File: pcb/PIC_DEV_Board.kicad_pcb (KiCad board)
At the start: 2 copper layers, 25.5 x 47.5 mm, 8 parts, among them J1 Conn_01x08_Pin, J3 Conn_01x15_Pin, J4 Conn_01x02_Pin

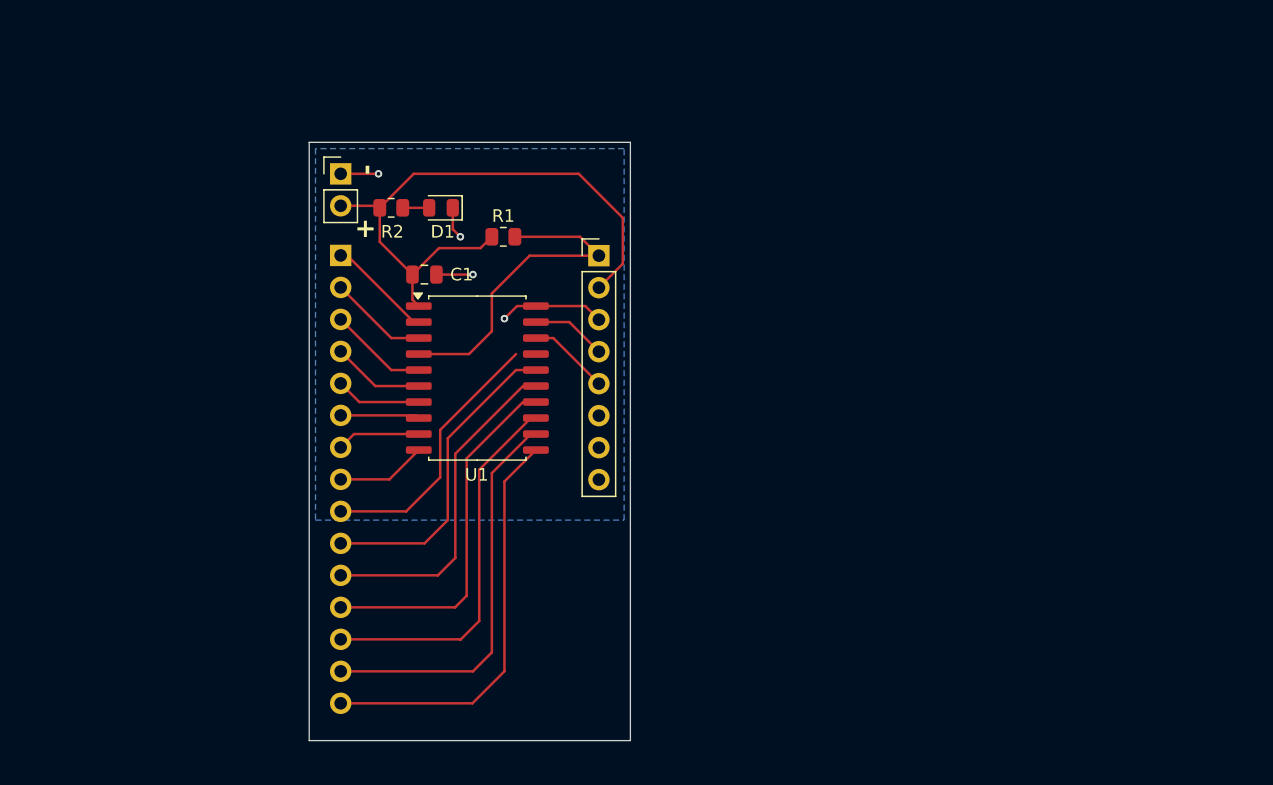
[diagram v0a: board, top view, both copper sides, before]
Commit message: higher functionality board
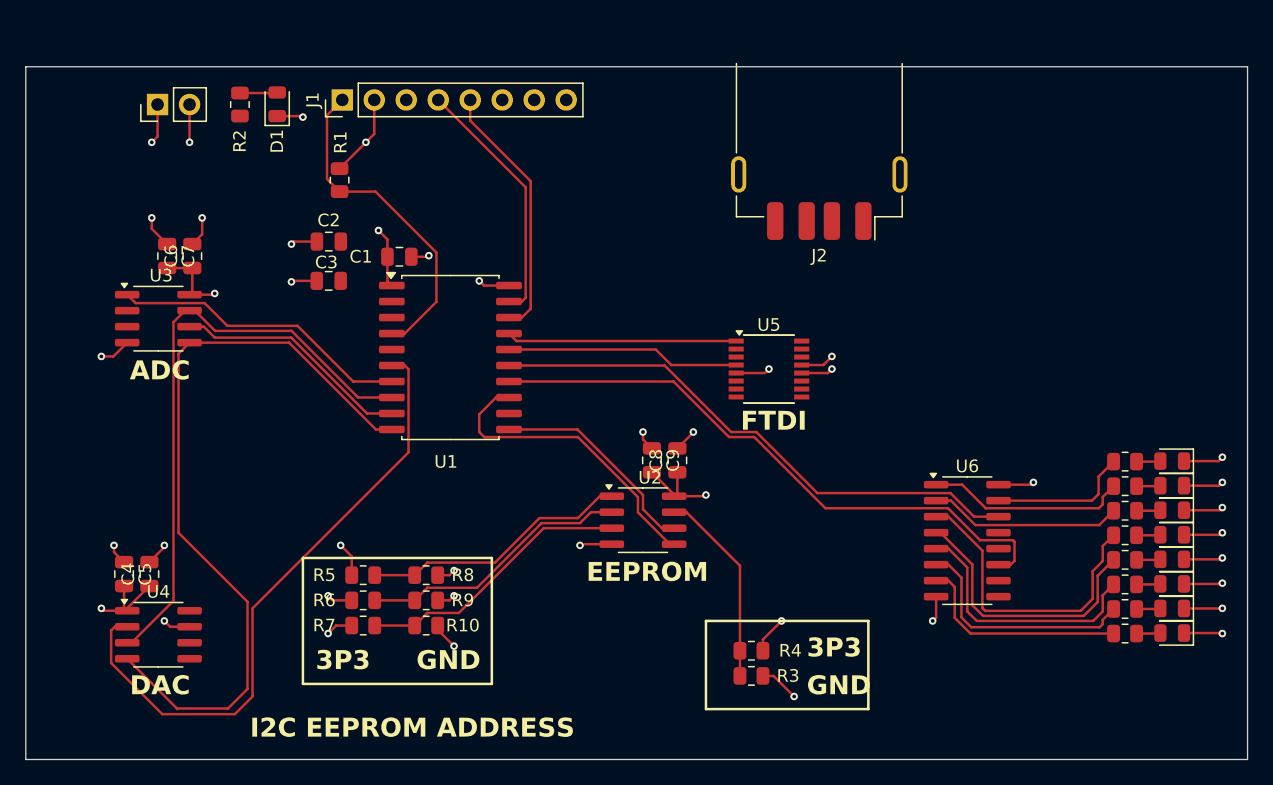
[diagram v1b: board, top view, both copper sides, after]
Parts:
- removed J3: Conn_01x15_Pin, Connector_PinHeader_2.54mm:PinHeader_1x15_P2.54mm_Vertical
- added C2: 30pF, Capacitor_SMD:C_0805_2012Metric, F.Cu at (136.1, 91.9)
- added C3: 30pF, Capacitor_SMD:C_0805_2012Metric, F.Cu at (136.1, 95.0)
- added C4: 0.1uF, Capacitor_SMD:C_0805_2012Metric, F.Cu at (121.8, 118.3)
- added C5: 10uF, Capacitor_SMD:C_0805_2012Metric, F.Cu at (119.8, 118.3)
- added C6: 0.1uF, Capacitor_SMD:C_0805_2012Metric, F.Cu at (125.2, 93.0)
- added C7: 10uF, Capacitor_SMD:C_0805_2012Metric, F.Cu at (123.2, 93.0)
- added C8: 0.1uF, Capacitor_SMD:C_0805_2012Metric, F.Cu at (163.7, 109.2)
- added C9: 10uF, Capacitor_SMD:C_0805_2012Metric, F.Cu at (161.7, 109.2)
- added D2: LED, LED_SMD:LED_0805_2012Metric, F.Cu at (203.0, 109.3)
- added D3: LED, LED_SMD:LED_0805_2012Metric, F.Cu at (203.0, 111.3)
- added D4: LED, LED_SMD:LED_0805_2012Metric, F.Cu at (203.0, 113.2)
- added D5: LED, LED_SMD:LED_0805_2012Metric, F.Cu at (203.0, 115.2)
- added D6: LED, LED_SMD:LED_0805_2012Metric, F.Cu at (203.0, 117.1)
- added D7: LED, LED_SMD:LED_0805_2012Metric, F.Cu at (203.0, 119.1)
- added D8: LED, LED_SMD:LED_0805_2012Metric, F.Cu at (203.0, 121.0)
- added D9: LED, LED_SMD:LED_0805_2012Metric, F.Cu at (203.0, 123.0)
- added J2: USB_A, Connector_USB:USB_A_Receptacle_GCT_USB1046, F.Cu at (175.0, 83.0)
- added R10: 10K, Resistor_SMD:R_0805_2012Metric, F.Cu at (143.8, 122.4)
- added R11: 560, Resistor_SMD:R_0805_2012Metric, F.Cu at (199.3, 109.3)
- added R12: 560, Resistor_SMD:R_0805_2012Metric, F.Cu at (199.3, 111.3)
- added R13: 560, Resistor_SMD:R_0805_2012Metric, F.Cu at (199.3, 113.2)
- added R14: 560, Resistor_SMD:R_0805_2012Metric, F.Cu at (199.3, 115.2)
- added R15: 560, Resistor_SMD:R_0805_2012Metric, F.Cu at (199.3, 117.2)
- added R16: 560, Resistor_SMD:R_0805_2012Metric, F.Cu at (199.3, 119.1)
- added R17: 560, Resistor_SMD:R_0805_2012Metric, F.Cu at (199.3, 121.0)
- added R18: 560, Resistor_SMD:R_0805_2012Metric, F.Cu at (199.3, 123.0)
- added R3: 0, Resistor_SMD:R_0805_2012Metric, F.Cu at (169.6, 126.4)
- added R4: 10K, Resistor_SMD:R_0805_2012Metric, F.Cu at (169.6, 124.4)
- added R5: 10K, Resistor_SMD:R_0805_2012Metric, F.Cu at (138.8, 118.4)
- added R6: 10K, Resistor_SMD:R_0805_2012Metric, F.Cu at (138.8, 120.4)
- added R7: 10K, Resistor_SMD:R_0805_2012Metric, F.Cu at (138.8, 122.4)
- added R8: 10K, Resistor_SMD:R_0805_2012Metric, F.Cu at (143.8, 118.4)
- added R9: 10K, Resistor_SMD:R_0805_2012Metric, F.Cu at (143.8, 120.4)
- added U2: ~, Package_SO:SOIC-8_3.9x4.9mm_P1.27mm, F.Cu at (161.0, 114.0)
- added U3: MCP3002, Package_SO:SOIC-8_3.9x4.9mm_P1.27mm, F.Cu at (122.5, 98.0)
- added U4: MCP4801, Package_SO:SOIC-8_3.9x4.9mm_P1.27mm, F.Cu at (122.5, 123.1)
- added U5: FT230XS, Package_SO:SSOP-16_3.9x4.9mm_P0.635mm, F.Cu at (171.0, 102.0)
- added U6: 74HC595, Package_SO:SOIC-16_3.9x9.9mm_P1.27mm, F.Cu at (186.8, 115.6)
- moved J1 23.8 mm to (137.1, 80.6), turned to 90 degrees
- moved J4 15.5 mm to (122.5, 81.0), turned to 90 degrees
- moved D1 15.4 mm to (132.0, 81.0), turned to 90 degrees
- moved R2 14.5 mm to (129.0, 81.0), turned to 90 degrees
- moved R1 13.8 mm to (136.9, 87.0), turned to -90 degrees
- moved U1 2.69 mm to (145.7, 101.1)
- moved C1 2.44 mm to (141.7, 93.1)
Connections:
- net Net-(J1-Pin_1) renamed /Vpp/RA3/MCLR
- net Net-(J1-Pin_2) renamed +3V3
- U1 pad 10: Net-(J3-Pin_8) -> /SDI
- U1 pad 12: Net-(J3-Pin_14) -> unconnected-(U1-RB5-Pad12)
- U1 pad 5: Net-(J3-Pin_3) -> unconnected-(U1-RC5-Pad5)
- U1 pad 6: Net-(J3-Pin_4) -> /~{DAC_CS}
- U1 pad 7: Net-(J3-Pin_5) -> /~{ADC_CS}
- U1 pad 8: Net-(J3-Pin_6) -> /SCK
- U1 pad 9: Net-(J3-Pin_7) -> /SDO
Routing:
- net /SDI: track 0.00 -> 60.9 mm
- net Earth: track 16.8 -> 73.0 mm, vias 4 -> 30
- net /~{DAC_CS}: track 0.00 -> 50.0 mm
- net /SCK: track 0.00 -> 47.7 mm
- net Net-(J3-Pin_14): track 31.6 -> 0.00 mm
- net Net-(U6-QD): track 0.00 -> 24.3 mm
- net /~{ADC_CS}: track 0.00 -> 23.9 mm
- net Net-(U2-A2): track 0.00 -> 22.0 mm
- net Net-(U6-QE): track 0.00 -> 21.8 mm
- net Net-(U2-A1): track 0.00 -> 21.7 mm
- net Net-(U2-A0): track 0.00 -> 21.4 mm
- net Net-(U6-QF): track 0.00 -> 20.5 mm
- net Net-(U1-RC2): track 28.6 -> 48.3 mm
- net /SDO: track 0.00 -> 18.9 mm
- net Net-(U6-QG): track 0.00 -> 18.8 mm
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- added copper zone on In2.Cu, net +3V3
- added copper zone on In1.Cu, net Earth
- removed copper zone on B.Cu, net Earth
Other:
- board size 25.5 x 47.5 mm -> 97 x 55 mm
- copper layers 2 -> 4
- board text added: "3P3"
- board text added: "ADC"
- board text added: "DAC"
- board text added: "EEPROM"
- board text added: "FTDI"
- board text added: "GND"
- board text added: "I2C EEPROM ADDRESS"
- board text removed: "+"
- board text removed: "-"

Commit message: size reduction
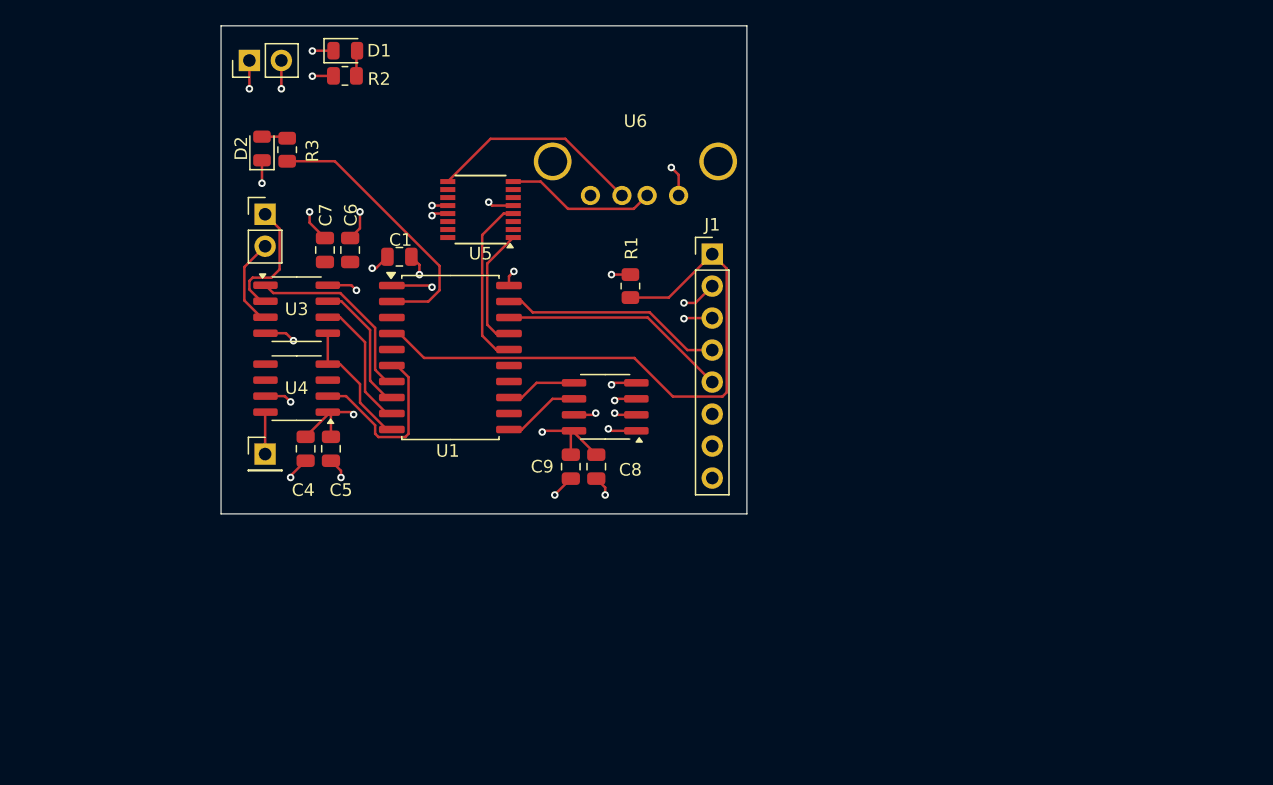
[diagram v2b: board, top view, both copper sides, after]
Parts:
- removed C2, C3: 30pF, Capacitor_SMD:C_0805_2012Metric
- removed D3, D4, D5, D6, D7, D8, D9: LED, LED_SMD:LED_0805_2012Metric
- removed J2: USB_A, Connector_USB:USB_A_Receptacle_GCT_USB1046
- removed R10, R4, R5, R6, R7, R8, R9: 10K, Resistor_SMD:R_0805_2012Metric
- removed R11, R12, R13, R14, R15, R16, R17, R18: 560, Resistor_SMD:R_0805_2012Metric
- added J3: Conn_01x02_Pin, Connector_PinHeader_2.54mm:PinHeader_1x02_P2.54mm_Vertical, F.Cu at (131.0, 89.7)
- added J5: Conn_01x01_Pin, Connector_PinHeader_2.54mm:PinHeader_1x01_P2.54mm_Vertical, F.Cu at (131.0, 108.8)
- R3: value 0 -> 1K
- U6: value 74HC595 -> ~; footprint Package_SO:SOIC-16_3.9x9.9mm_P1.27mm -> myCustomFootprints:USB-A1HSB6
- moved D2 76.4 mm to (130.8, 84.5), turned to 90 degrees
- moved R3 55.7 mm to (132.8, 84.6), turned to 90 degrees
- moved U6 38.1 mm to (160.3, 88.2), turned to 180 degrees
- moved J1 31.8 mm to (166.5, 92.9), turned to 0 degrees
- moved U5 26.2 mm to (148.1, 89.3), turned to 180 degrees
- moved R1 24.6 mm to (160.0, 95.4)
- moved U4 22.4 mm to (133.5, 103.5), turned to 180 degrees
- moved C5 19.2 mm to (136.2, 108.3), turned to 90 degrees
- moved C4 15.9 mm to (134.2, 108.3), turned to -90 degrees
- moved C6 12.5 mm to (137.8, 92.5)
- moved C7 12.5 mm to (135.8, 92.5)
- moved U3 11.0 mm to (133.5, 97.2)
- moved U2 9.49 mm to (158.0, 105.0), turned to 180 degrees
- moved R2 8.64 mm to (137.3, 78.7), turned to 0 degrees
- moved C8 8.47 mm to (155.3, 109.8), turned to -90 degrees
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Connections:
- R3 pad 1: Earth -> Net-(U1-RA5)
- R3 pad 2: Net-(U2-WP) -> Net-(D2-A)
- U1 pad 14: Net-(U1-RC2) -> unconnected-(U1-RC2-Pad14)
- U1 pad 15: Net-(U1-RC1) -> unconnected-(U1-RC1-Pad15)
- U1 pad 3: Net-(U1-RA4) -> unconnected-(U1-RA4-Pad3)
- U2 pad 1: Net-(U2-A0) -> Earth
- U2 pad 2: Net-(U2-A1) -> Earth
- U2 pad 3: Net-(U2-A2) -> Earth
- U2 pad 7: Net-(U2-WP) -> Earth
- U3 pad 2: unconnected-(U3-CH0-Pad2) -> Net-(J3-Pin_1)
- U3 pad 3: unconnected-(U3-CH1-Pad3) -> Net-(J3-Pin_2)
- U4 pad 8: unconnected-(U4-Vout-Pad8) -> Net-(J5-Pin_1)
- U5 pad 8: Net-(J2-D+) -> Net-(U5-USBDP)
- U5 pad 9: Net-(J2-D-) -> Net-(U5-USBDM)
- U6 pad 1: Net-(U6-QB) -> unconnected-(U6-VCC-Pad1)
- U6 pad 2: Net-(U6-QC) -> Net-(U5-USBDM)
- U6 pad 3: Net-(U6-QD) -> Net-(U5-USBDP)
- U6 pad 4: Net-(U6-QE) -> Earth
- U6 pad 5: Net-(U6-QF) -> (no net)
- U6 pad 6: Net-(U6-QG) -> (no net)
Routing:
- net /SDI: track 60.9 -> 10.6 mm
- net Net-(U1-RC2): track 48.3 -> 0.00 mm
- net Net-(U1-RC1): track 43.8 -> 0.00 mm
- net /SCK: track 47.7 -> 10.6 mm
- net /~{DAC_CS}: track 50.0 -> 14.5 mm
- net Earth: track 73.0 -> 43.1 mm, vias 30 -> 22
- net Net-(U6-QD): track 24.3 -> 0.00 mm
- net Net-(U2-A2): track 22.0 -> 0.00 mm
- net /Vpp/RA3/MCLR: track 26.4 -> 48.2 mm
- net Net-(U6-QE): track 21.8 -> 0.00 mm
- net Net-(U2-A1): track 21.7 -> 0.00 mm
- net Net-(U1-RA5): track 0.00 -> 21.6 mm
- net Net-(U2-A0): track 21.4 -> 0.00 mm
- net Net-(U6-QF): track 20.5 -> 0.00 mm
- net +3V3: track 50.0 -> 30.8 mm, vias 12 -> 10
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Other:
- board size 97 x 55 mm -> 41.8 x 38.8 mm
- board text removed: "3P3"
- board text removed: "ADC"
- board text removed: "DAC"
- board text removed: "EEPROM"
- board text removed: "FTDI"
- board text removed: "GND"
- board text removed: "I2C EEPROM ADDRESS"
